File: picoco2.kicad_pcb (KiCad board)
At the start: 2 copper layers, 54.5 x 103.4 mm, 41 parts, among them J1 Conn_01x03_Female, J2 Micro_SD_Card, J3 Conn_01x03_Female, Q1 Q_NMOS_GDS, SW1 SW_Push, SW2 SW_Push, U1 PicoW, U2 scd30, U3 ssd1306, U4 PCF8523T, U5 MCP73831-2-OT, Y1 Crystal_GND23

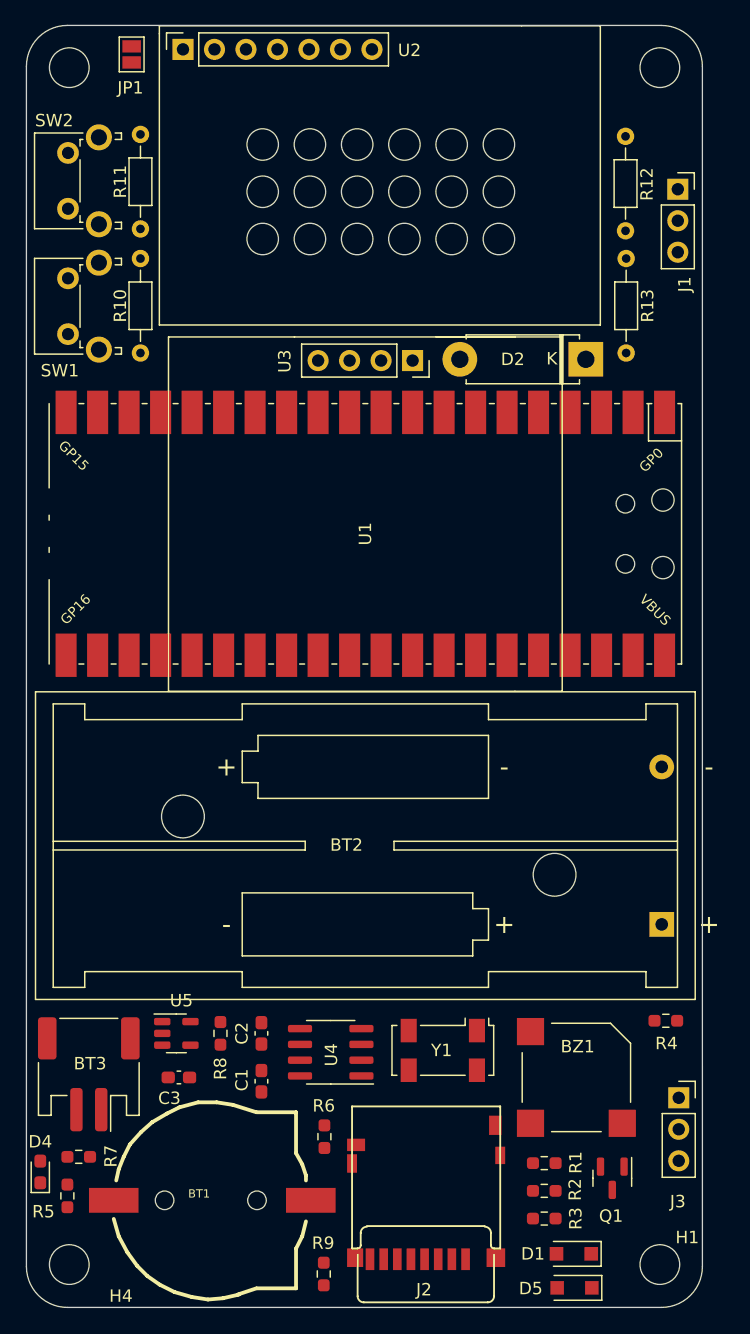
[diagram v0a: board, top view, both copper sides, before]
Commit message: update
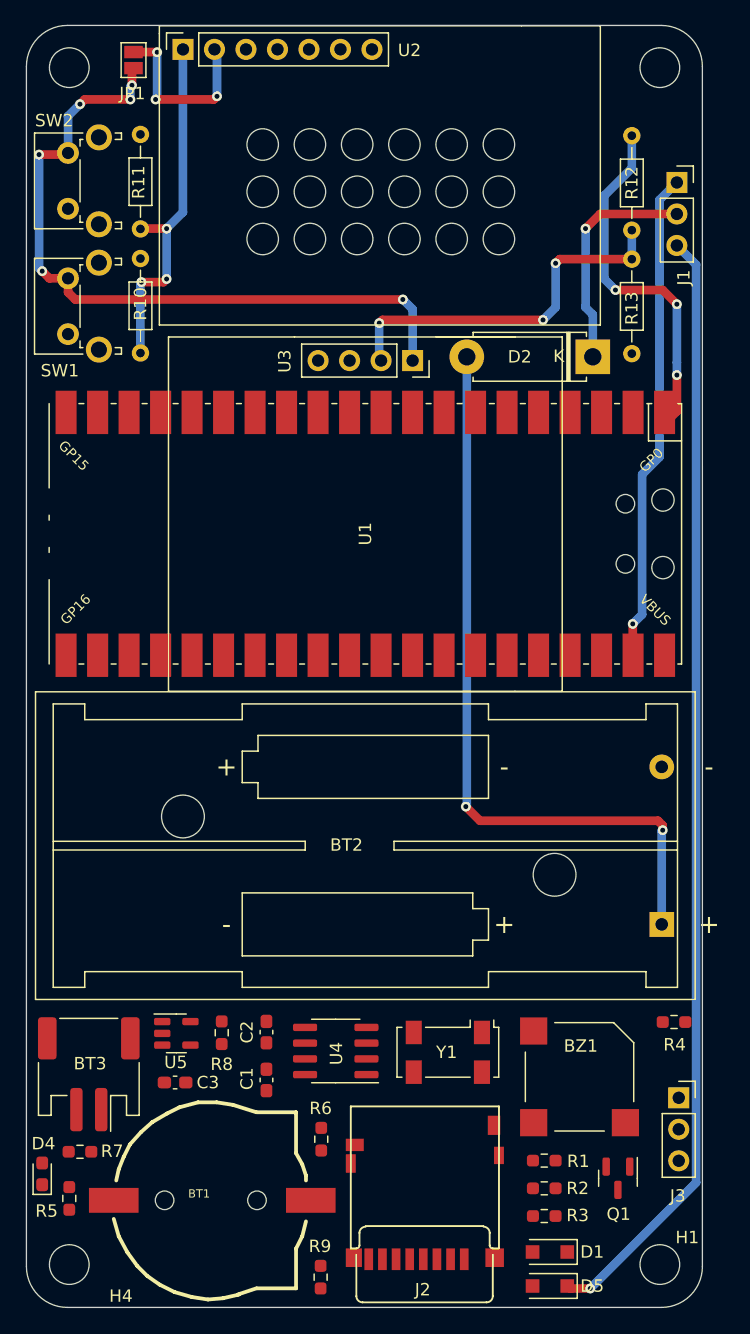
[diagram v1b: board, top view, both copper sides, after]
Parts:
- moved R13 7.58 mm to (48.8, 18.8), turned to -90 degrees
- moved D5 1.99 mm to (42.2, 101.7)
- moved D1 1.94 mm to (42.2, 98.9)
- moved R4 0.67 mm to (52.2, 80.4)
- moved D2 0.59 mm to (45.7, 26.7)
- moved J1 0.55 mm to (52.5, 12.7)
- moved R12 0.51 mm to (48.8, 16.5)
- moved C3 0.51 mm to (12.0, 85.2)
- moved JP1 0.48 mm to (8.64, 2.79)
- moved Q1 0.46 mm to (47.7, 93.0)
- moved Y1 0.43 mm to (34.0, 82.8)
- moved R7 0.42 mm to (4.32, 90.8)
- moved C1 0.42 mm to (19.4, 85.0)
- moved C2 0.42 mm to (19.4, 81.2)
- moved U4 0.42 mm to (24.9, 82.7)
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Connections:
- U2 pad 4: SCL -> SDA
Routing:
- net Net-(D5-Pad1): track 0.00 -> 90.2 mm, vias 0 -> 1
- net VBAT_AAA: track 0.00 -> 60.8 mm, vias 0 -> 2
- net +3V3: track 0.00 -> 59.1 mm, vias 0 -> 6
- net GND: track 0.00 -> 59.0 mm, vias 0 -> 6
- net VSYS: track 0.00 -> 38.7 mm, vias 0 -> 1
- net SDA: track 0.00 -> 29.2 mm, vias 0 -> 3
- net Net-(D1-Pad1): track 0.00 -> 18.4 mm, vias 0 -> 1
- net SCD30_GND: track 0.00 -> 14.7 mm, vias 0 -> 3
